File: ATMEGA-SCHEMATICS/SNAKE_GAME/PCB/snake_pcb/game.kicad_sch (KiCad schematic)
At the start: 29 parts, among them J10 LCD_SCREEN, J14 Conn_01x05_Pin, J15 Conn_01x04_Pin, J17 Conn_01x06_Pin, J19 Conn_01x06_Pin, J6 TERM_GAME, J8 Conn_01x03_Pin, J9 Conn_01x05_Pin, U2 ATmega168A-P, Y2 Crystal

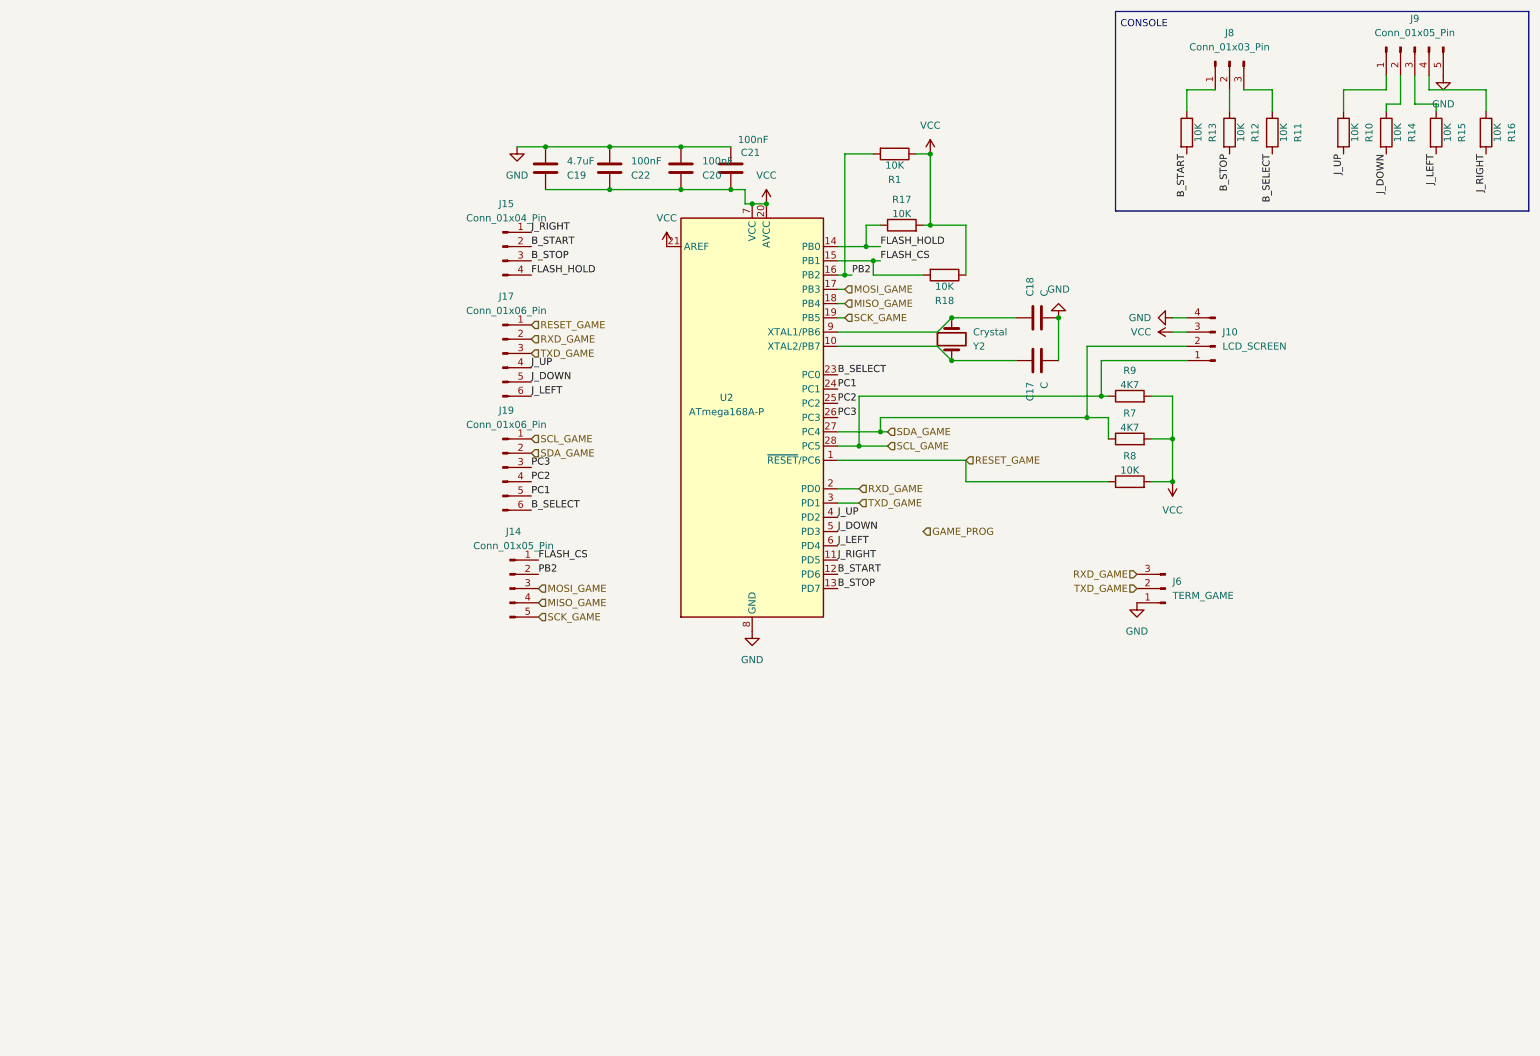
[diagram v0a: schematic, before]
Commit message: ...
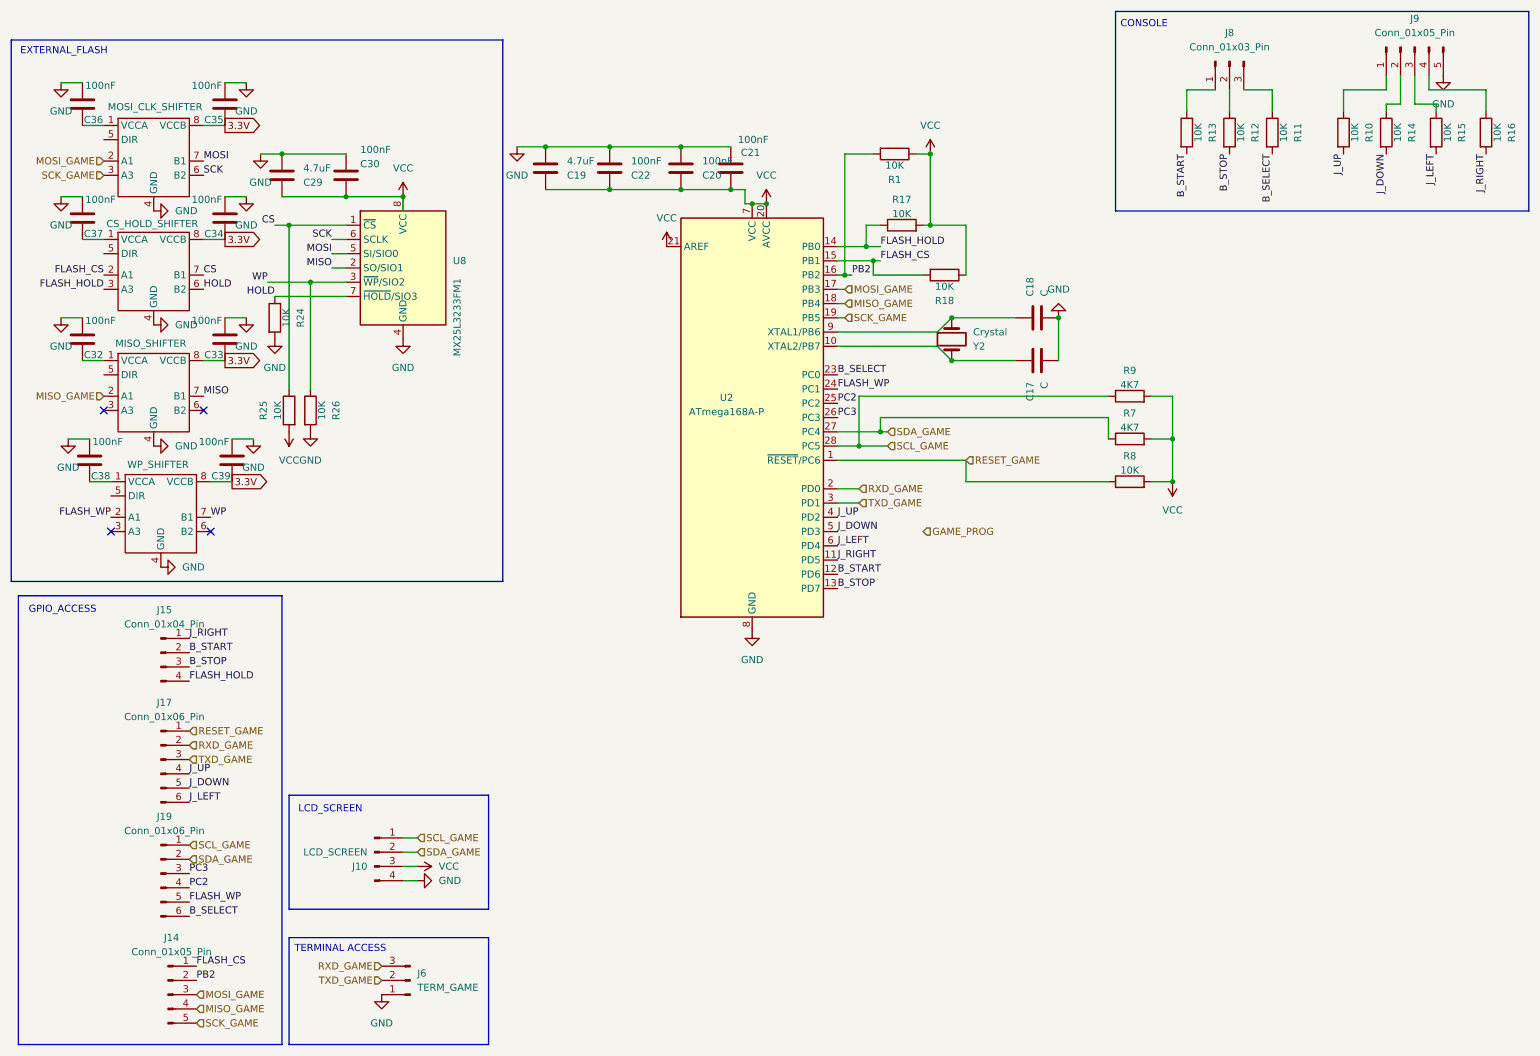
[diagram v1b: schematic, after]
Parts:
- added C29: 4.7uF, symbol Device:C
- added C30, C32, C33, C34, C35, C36, C37, C38, C39: 100nF, symbol Device:C
- added CS_HOLD_SHIFTER, MISO_SHIFTER, MOSI_CLK_SHIFTER, WP_SHIFTER: ~, symbol lucasLib:SN74LXC2T45
- added R24, R25, R26: 10K, symbol Device:R
- added U8: MX25L3233FM1, Package_SO:SOP-8_3.9x4.9mm_P1.27mm, symbol Memory_Flash:MX25L3233FM1
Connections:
- net FLASH_CS: now also CS_HOLD_SHIFTER.2 (A1)
- net FLASH_HOLD: now also CS_HOLD_SHIFTER.3 (A3)
- net GND: now also C29.2, C30.2, C32.2, C33.2, C34.2, C35.2, C36.2, C37.2, C38.2, C39.2, CS_HOLD_SHIFTER.4 (GND), MISO_SHIFTER.4 (GND), MOSI_CLK_SHIFTER.4 (GND), R24.2, R26.2, U8.4 (GND), WP_SHIFTER.4 (GND)
- net MISO_GAME: now also MISO_SHIFTER.2 (A1)
- net MOSI_GAME: now also MOSI_CLK_SHIFTER.2 (A1)
- net SCK_GAME: now also MOSI_CLK_SHIFTER.3 (A3)
- net VCC: now also C29.1, C30.1, R25.2, U8.8 (VCC)
- net PC1 renamed FLASH_WP
- net FLASH_WP: now also WP_SHIFTER.2 (A1)
- new net: C38.1, WP_SHIFTER.1 (VCCA)
- new net: C32.1, MISO_SHIFTER.1 (VCCA)
- new net: C36.1, MOSI_CLK_SHIFTER.1 (VCCA)
- new net: C37.1, CS_HOLD_SHIFTER.1 (VCCA)
- new net 3.3V: C33.1, C34.1, C35.1, C39.1, CS_HOLD_SHIFTER.8 (VCCB), MISO_SHIFTER.8 (VCCB), MOSI_CLK_SHIFTER.8 (VCCB), WP_SHIFTER.8 (VCCB)
- new net CS: CS_HOLD_SHIFTER.7 (B1), R25.1, U8.1 (~{CS})
- new net HOLD: CS_HOLD_SHIFTER.6 (B2), R24.1, U8.7 (~{HOLD}/SIO3)
- new net MISO: MISO_SHIFTER.7 (B1), U8.2 (SO/SIO1)
- new net MOSI: MOSI_CLK_SHIFTER.7 (B1), U8.5 (SI/SIO0)
- new net SCK: MOSI_CLK_SHIFTER.6 (B2), U8.6 (SCLK)
- new net WP: R26.1, U8.3 (~{WP}/SIO2), WP_SHIFTER.7 (B1)
- no-connect marks 0 -> 4
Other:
- note added: "EXTERNAL_FLASH"
- note added: "GPIO_ACCESS"
- note added: "LCD_SCREEN"
- note added: "TERMINAL ACCESS"
- moved on the sheet: J10, J14, J15, J17, J19, J6
